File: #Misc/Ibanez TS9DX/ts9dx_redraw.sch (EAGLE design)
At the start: 73 parts, among them IC101 RC4558, Q101 2SC1815BL, Q102 1SK44SP, Q103 2SC1815BL, Q104 2SK44SP, Q105 2SC1815BL, Q106 2SC1815BL, Q107 2SC1815BL

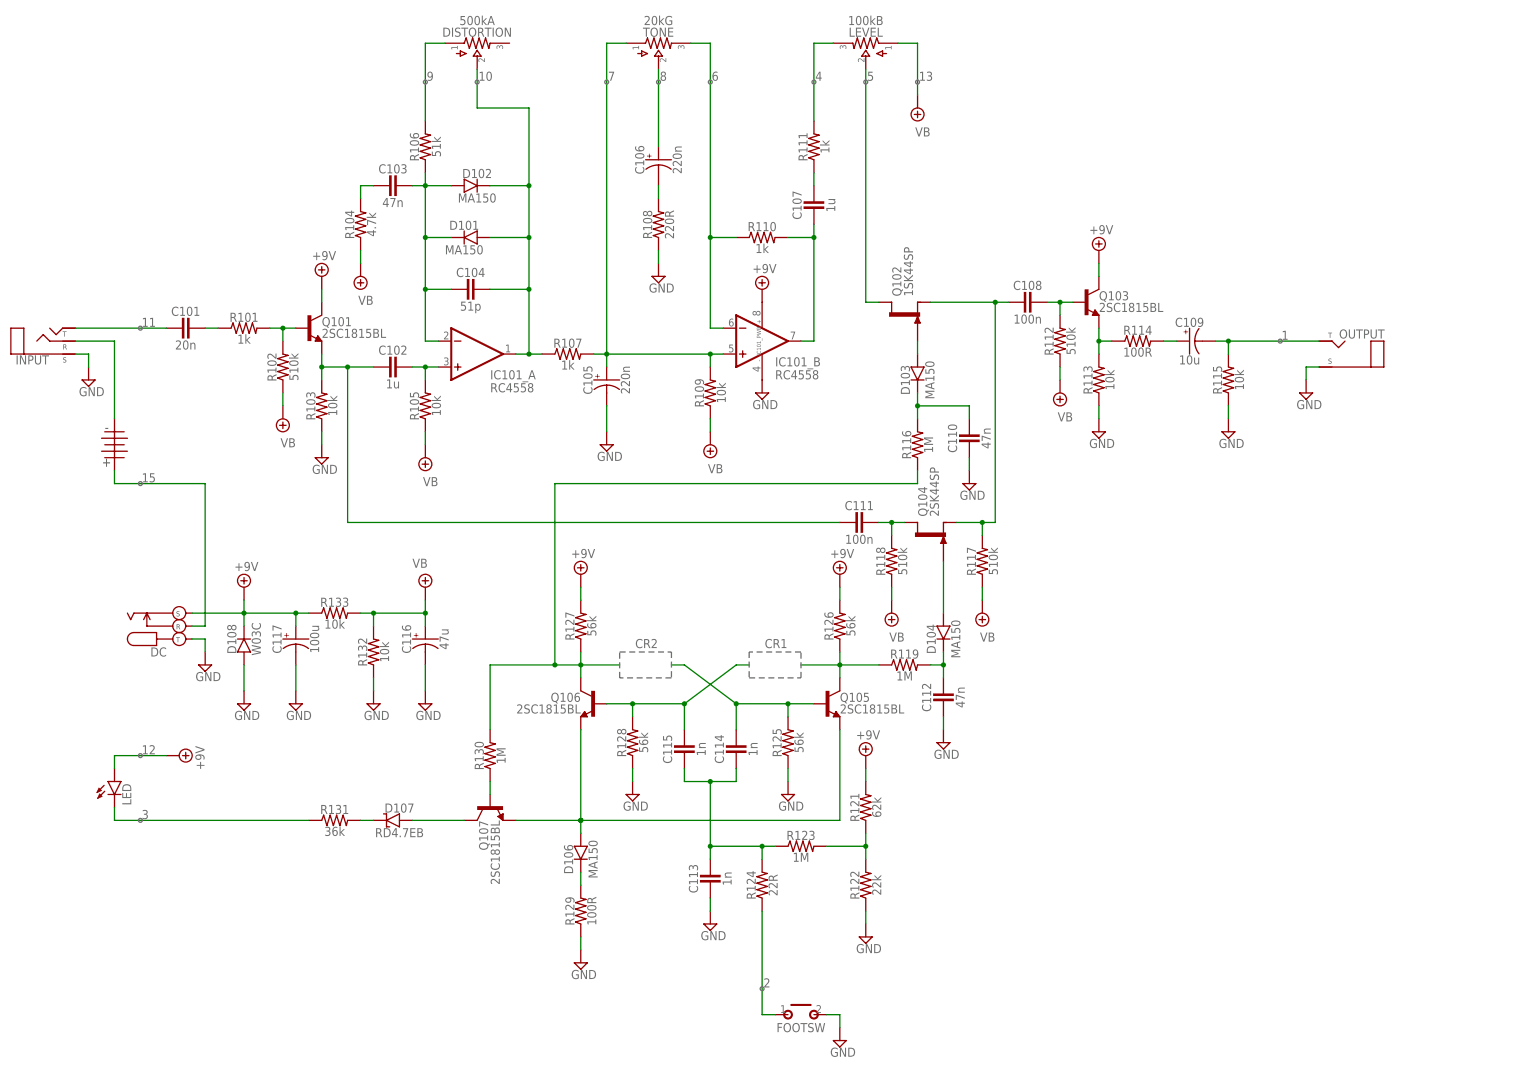
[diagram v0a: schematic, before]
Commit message: 20200325/10:41
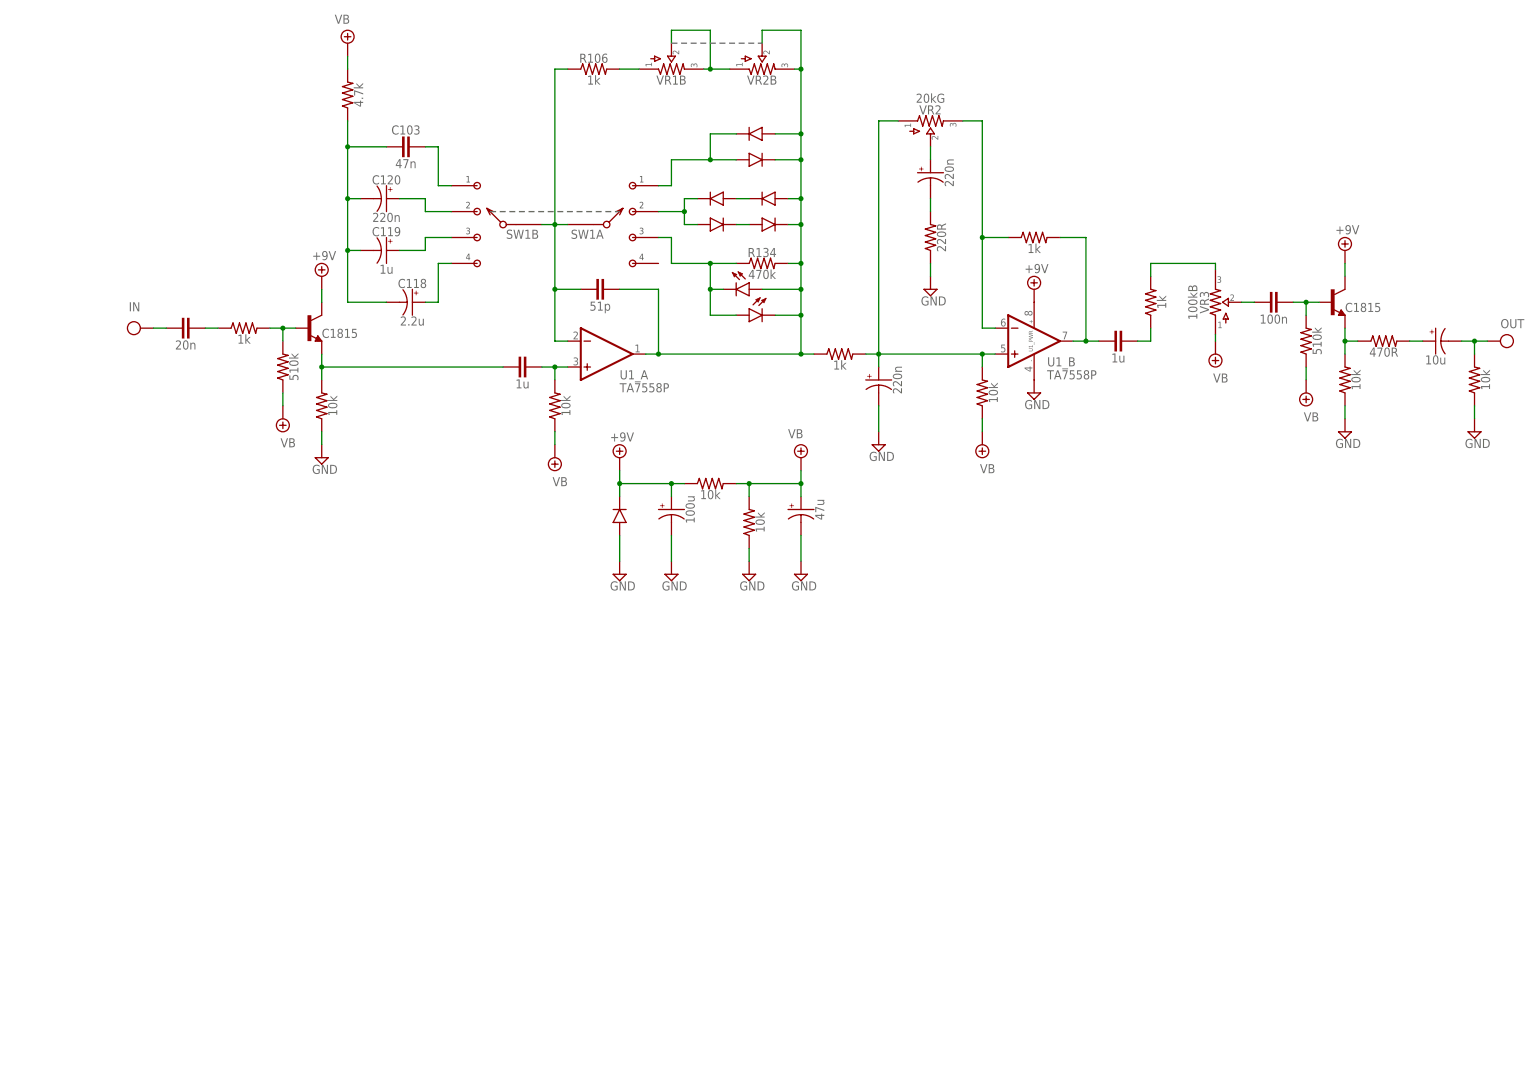
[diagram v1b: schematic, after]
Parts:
- removed BATTERY: BATTERY, pedals-jacks:BATTERY
- removed C104: 51p, pedals-capacitors-film:CER/FILMBOX.1
- removed C110, C112: 47n, pedals-capacitors-film:CER/FILMBOX.1
- removed C111: 100n, pedals-capacitors-film:CER/FILMBOX.1
- removed C113, C114, C115: 1n, pedals-capacitors-film:CER/FILMBOX.1
- removed D101, D102, D103, D104, D106: MA150, pedals-diodes:DO35.2
- removed D107: RD4.7EB, pedals-diodes:ZENER.2
- removed DC: DCJACK, pedals-jacks:DC_KOBICONN
- removed DISTORTION: 500kA, pedals-potentiometers:POTS16MM
- removed FOOTSW: MOMENTARY, pedals-switches:MOMENTARY
- removed IC101: RC4558, pedals-integrated circuits:DUALTH
- removed INPUT: (no value), pedals-jacks:STEREO3PADS
- removed LED: LED, pedals-diodes:LED
- removed LEVEL: 100kB, pedals-potentiometers:POTS16MM
- removed OUTPUT: (no value), pedals-jacks:MONO
- removed Q102: 1SK44SP, pedals-transistors:2N5457
- removed Q104: 2SK44SP, pedals-transistors:2N5457
- removed Q105, Q106, Q107: 2SC1815BL, pedals-transistors:2SC828A
- removed R104: 4.7k, pedals-resistors:R_.3B
- removed R116, R119, R123, R130: 1M, pedals-resistors:R_.3B
- removed R117, R118: 510k, pedals-resistors:R_.3B
- removed R121: 62k, pedals-resistors:R_.3B
- removed R122: 22k, pedals-resistors:R_.3B
- removed R124: 22R, pedals-resistors:R_.3B
- removed R125, R126, R127, R128: 56k, pedals-resistors:R_.3B
- removed R129: 100R, pedals-resistors:R_.3B
- removed R131: 36k, pedals-resistors:R_.3B
- removed TONE: 20kG, pedals-potentiometers:POTS16MM
- added C1: 51p, pedals-capacitors-film:CER/FILMBOX.1
- added C118: 2.2u, pedals-capacitors-elec:0500
- added C119: 1u, pedals-capacitors-elec:0500
- added C120: 220n, pedals-capacitors-elec:0500
- added D1, D2, D3, D4, D7, D8: (no value), pedals-diodes:DO35.2
- added D5, D6: LED, pedals-diodes:LED
- added R134: 470k, pedals-resistors:R_.3B
- added R3: 4.7k, pedals-resistors:R_.3B
- added SW1: (no value), pedals-switches:2P4T
- added U1: TA7558P, pedals-integrated circuits:DUALTH
- added VR1B, VR2B: (no value), pedals-potentiometers:POTS16MM
- added VR2: 20kG, pedals-potentiometers:POTS16MM
- added VR3: 100kB, pedals-potentiometers:POTS16MM
- D108: value W03C -> (none)
- Q101, Q103: value 2SC1815BL -> C1815
- R106: value 51k -> 1k
- R114: value 100R -> 470R
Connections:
- removed net N$2 (its old number): BATTERY.P$2, INPUT.R
- removed net N$29: Q106.C, R116.1, R127.1, R130.2
- removed net N$30: Q107.B, R130.1
- removed net N$31: Q105.C, R119.1, R126.1
- removed net N$32: C115.1, Q106.B, R128.2
- removed net N$34: C114.1, Q105.B, R125.2
- removed net N$35: D106.A, Q105.E, Q106.E, Q107.E
- removed net N$36: C113.1, C114.2, C115.2, R123.1, R124.2
- removed net N$37: D106.C, R129.2
- removed net N$38: R121.1, R122.2, R123.2
- removed net N$39: FOOTSW.P, R124.1
- removed net N$40: LED.C, R131.1
- removed net N$41: D107.C, R131.2
- removed net N$42: D107.A, Q107.C
- new net IN: C101.2
- new net N$13: C1.2, R106.1, SW1A.A, SW1B.A, U1_A.-IN
- new net OUT: C109.-, R115.2
- net +9V: now also U1_PWR.V+; no longer DC.S, IC101_PWR.V+, LED.A, R121.2, R126.2, R127.2
- net GND: now also U1_PWR.V-; no longer C110.2, C112.2, C113.2, DC.T, FOOTSW.S, IC101_PWR.V-, INPUT.S, OUTPUT.SLEEVE, R122.1, R125.1, R128.1, R129.1
- net N$1: now also D1.A, D4.C, SW1A.2; no longer C101.2, INPUT.T
- net N$10: now also U1_B.+IN, VR2.1; no longer IC101_B.+IN, TONE.1
- net N$11: now also U1_B.-IN, VR2.3; no longer IC101_B.-IN, TONE.3
- net N$12: now also U1_B.OUT; no longer IC101_B.OUT
- net N$14: now also VR2.2; no longer TONE.2
- net N$16: now also D7.A, D8.C, SW1A.1; no longer LEVEL.3, R111.2
- net N$17: now also C1.1, D2.C, D3.A, D5.A, D6.C, D7.C, D8.A, R107.1, R134.2, U1_A.OUT, VR2B.2, VR2B.3; no longer LEVEL.2, Q102.D
- net N$18: now also D5.C, D6.A, R134.1, SW1A.3; no longer C108.2, Q102.S, Q104.S, R117.2
- net N$19: now also VR1B.2, VR1B.3, VR2B.1; no longer D103.A, Q102.G
- net N$20: now also C108.2, VR3.2; no longer C110.1, D103.C, R116.2
- net N$21: now also C119.+, SW1B.3; no longer D104.A, Q104.G
- net N$22: now also C118.+, SW1B.4; no longer C112.1, D104.C, R119.2
- net N$26: now also C120.+, SW1B.2; no longer C109.-, OUTPUT.TIP, R115.2
- net N$27: now also C103.2, C118.-, C119.-, C120.-, R3.1; no longer C111.1, Q104.D, R118.2
- net N$28: now also C103.1, SW1B.1; no longer BATTERY.P$1, DC.R
- net N$4: no longer C111.2
- net N$5: now also U1_A.+IN; no longer IC101_A.+IN
- net N$6: now also D1.C, D2.A; no longer C103.1, C104.2, D101.C, D102.A, IC101_A.-IN, R106.1
- net N$7: now also R111.2, VR3.3; no longer DISTORTION.1, R106.2
- net N$8: now also R106.2, VR1B.1; no longer C104.1, D101.A, D102.C, DISTORTION.2, IC101_A.OUT, R107.1
- net N$9: now also D3.C, D4.A; no longer C103.2, R104.2
- net VB: now also R3.2, VR3.1; no longer LEVEL.1, R104.1, R117.1, R118.1
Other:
- note removed: "1"
- note removed: "10"
- note removed: "11"
- note removed: "12"
- note removed: "13"
- note removed: "15"
- note removed: "2"
- note removed: "3"
- note removed: "4"
- note removed: "5"
- note removed: "6"
- note removed: "7"
- note removed: "8"
- note removed: "9"
- note removed: "CR1"
- note removed: "CR2"
- moved on the sheet: C103, R106
